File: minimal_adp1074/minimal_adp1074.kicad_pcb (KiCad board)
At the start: 4 copper layers, 25.4 x 25.4 mm, 0 parts

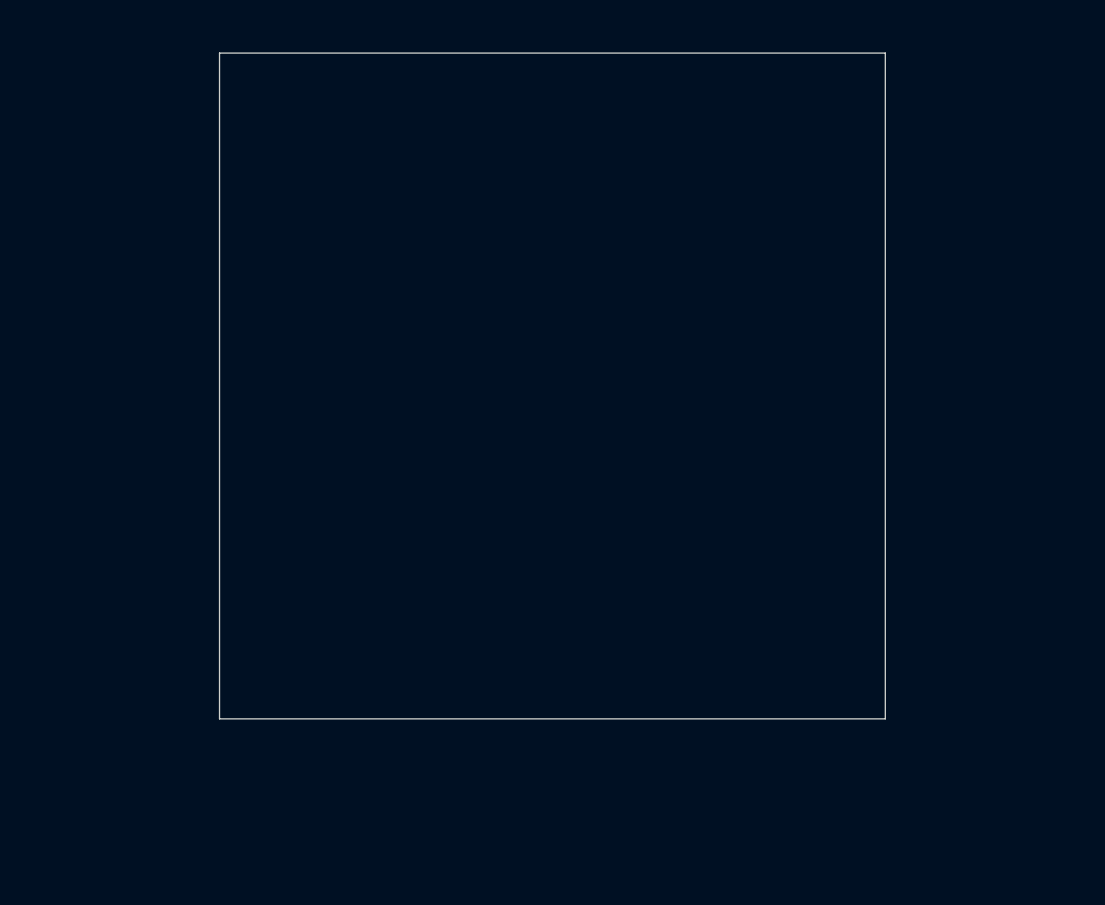
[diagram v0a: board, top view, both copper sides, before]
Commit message: backup
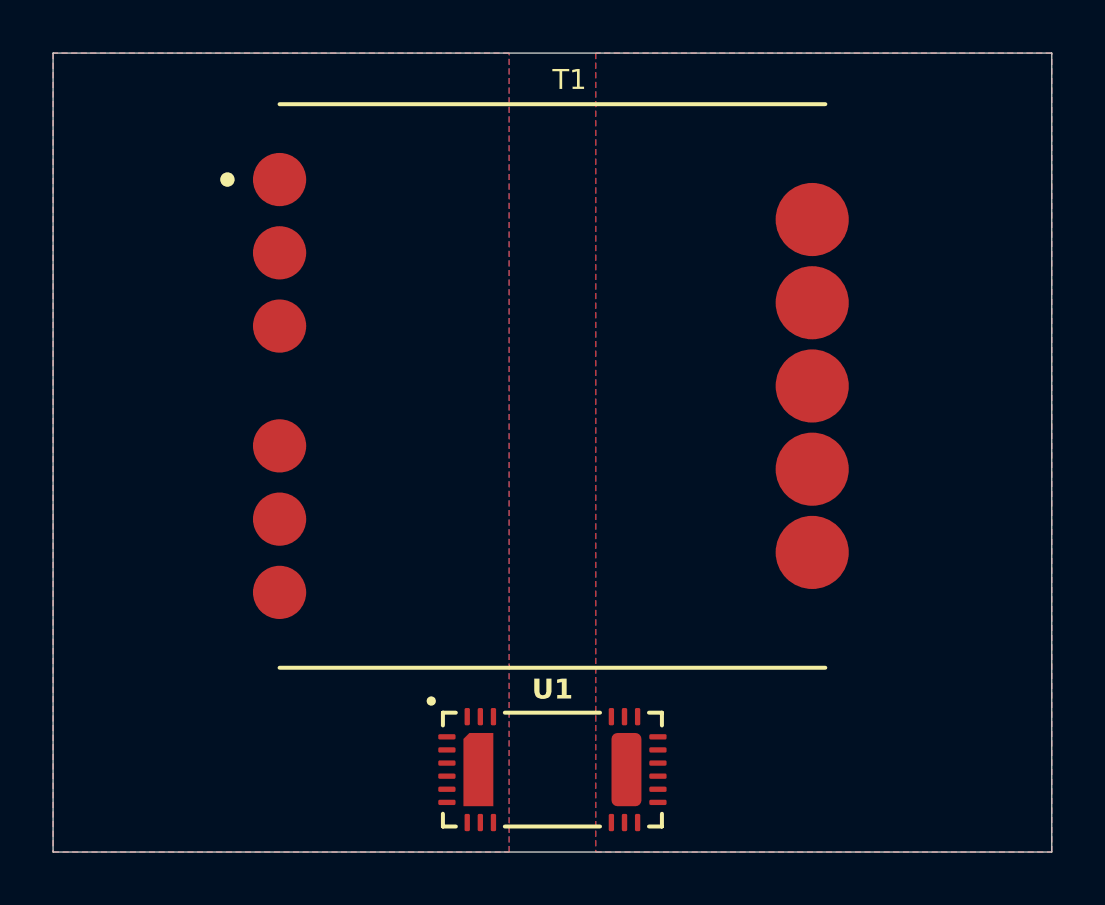
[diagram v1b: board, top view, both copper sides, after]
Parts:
- added T1: PL160X9-102L-BLD, transformer_footprints:PL160X9-102L, F.Cu at (152.4, 88.9)
- added U1: ADP1074ACCZ-R7, analog_devices_footprints:CC-24-6_ADI, F.Cu at (152.4, 103.5)
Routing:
- added copper zone on B.Cu, net GND
- added copper zone on F.Cu, net GND
- added copper zone on In1.Cu, net GND
- added copper zone on In2.Cu, net GND
- added copper zone on B.Cu, net GNDA
- added copper zone on F.Cu, net GNDA
- added copper zone on In1.Cu, net GNDA
- added copper zone on In2.Cu, net GNDA
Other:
- board size 25.4 x 25.4 mm -> 38.1 x 30.5 mm
